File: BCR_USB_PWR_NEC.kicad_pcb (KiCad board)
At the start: 2 copper layers, 13.4 x 21.8 mm, 2 parts, among them CN1 DB9_Female, CN2 UE27AC54100

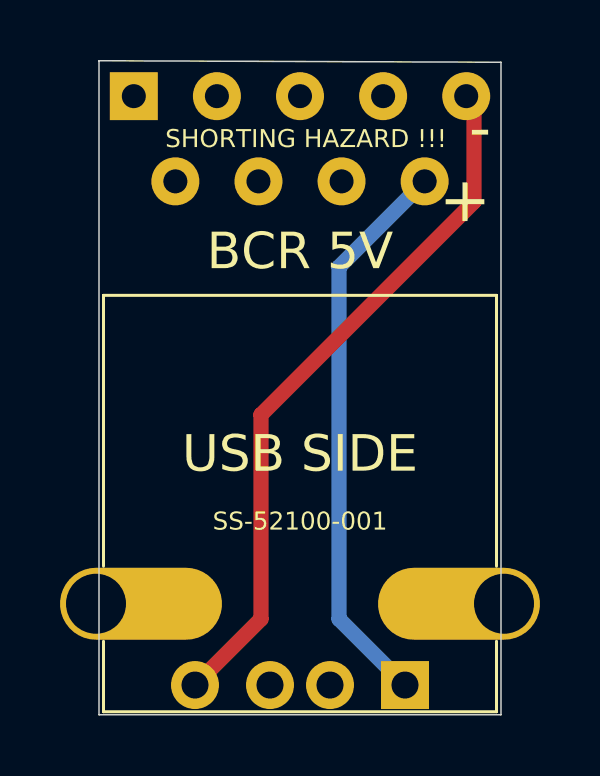
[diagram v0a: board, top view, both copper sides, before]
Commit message: clean up junk files
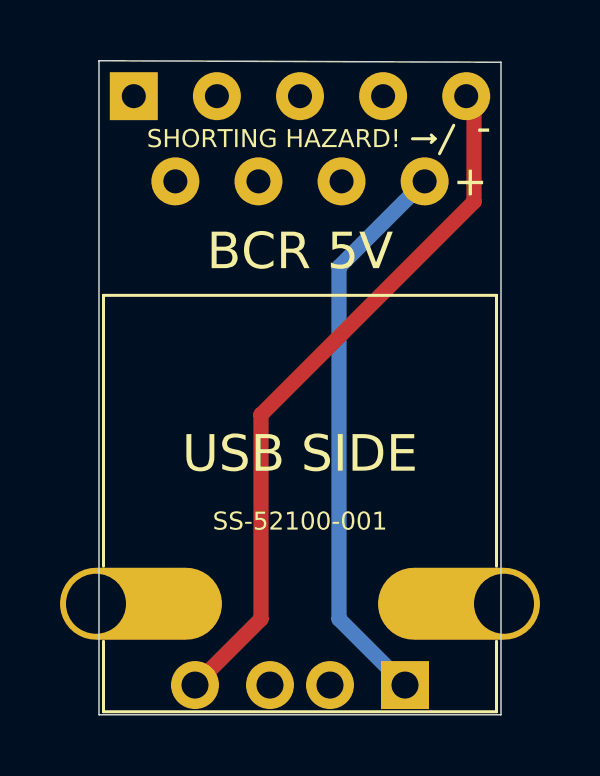
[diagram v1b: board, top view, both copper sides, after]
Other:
- board text added: "SHORTING HAZARD!"
- board text removed: "SHORTING HAZARD !!!"
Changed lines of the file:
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@@
   (general
     (thickness 1.6)
-    (drawings 20)
+    (drawings 24)
     (tracks 8)
     (zones 0)
@@
     )
   )
-  (gr_text "SHORTING HAZARD !!!" (at 127.2 95.758) (layer F.SilkS)
+  (gr_line (start 131.5 95.758) (end 131.375 95.633) (layer F.SilkS) (width 0.1016))
+  (gr_line (start 131.5 95.758) (end 131.375 95.883) (layer F.SilkS) (width 0.1016))
+  (gr_line (start 131.5 95.758) (end 130.75 95.758) (layer F.SilkS) (width 0.1016))
+  (gr_line (start 131.65 96.258) (end 132.125 95.308) (layer F.SilkS) (width 0.1016))
+  (gr_text "SHORTING HAZARD!" (at 126.125 95.758) (layer F.SilkS)
     (effects (font (size 0.6 0.6) (thickness 0.06)))
   )
-  (gr_text - (at 133 95.408) (layer F.SilkS)
-    (effects (font (size 1.5 1.5) (thickness 0.15)))
-  )
-  (gr_text + (at 132.5 97.808) (layer F.SilkS)
-    (effects (font (size 1.5 1.5) (thickness 0.15)))
+  (gr_text - (at 133.125 95.383) (layer F.SilkS)
+    (effects (font (size 1 1) (thickness 0.1)))
+  )
+  (gr_text + (at 132.675 97.183) (layer F.SilkS)
+    (effects (font (size 1 1) (thickness 0.1)))
   )
   (gr_text "A-DF 09 PP/Z" (at 127 95.758) (layer B.SilkS)
